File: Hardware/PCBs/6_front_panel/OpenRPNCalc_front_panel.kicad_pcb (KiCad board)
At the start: 2 copper layers, 73 x 134.4 mm, 1 part

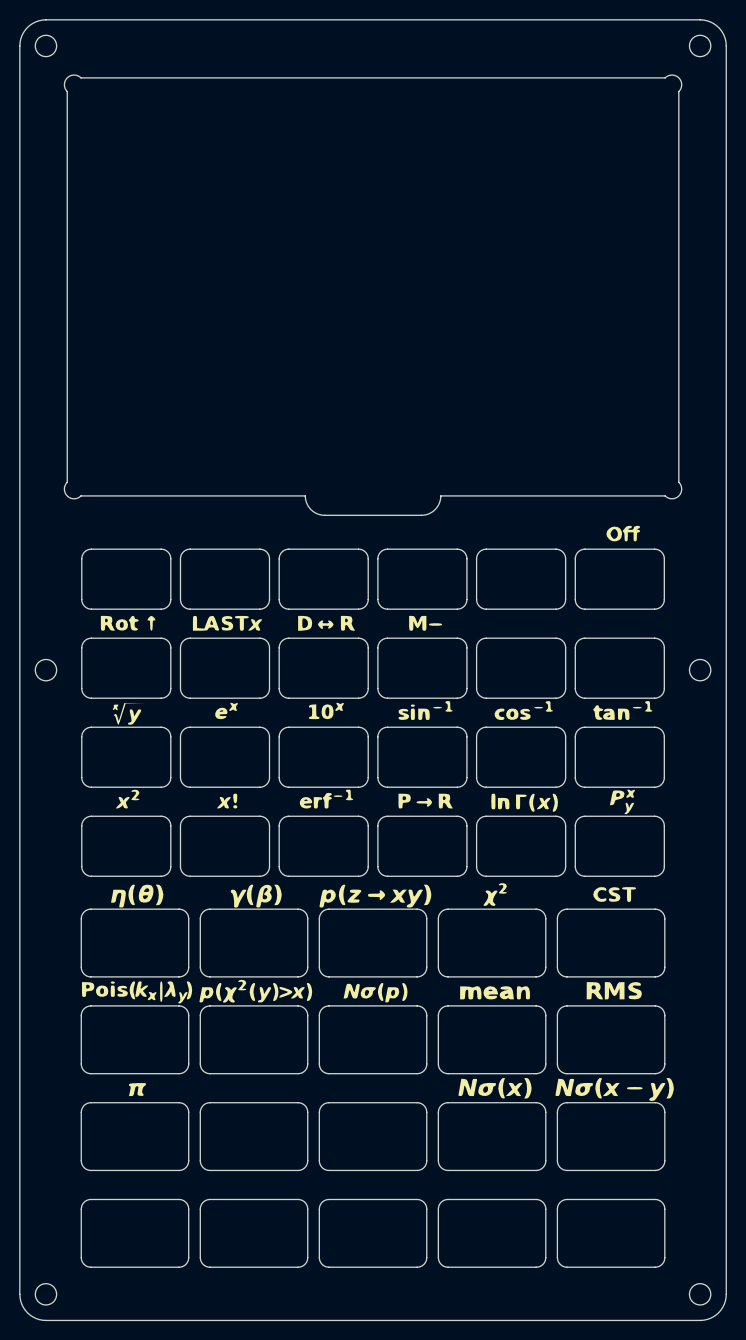
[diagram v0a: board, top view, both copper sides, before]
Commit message: Update to rev 3.1
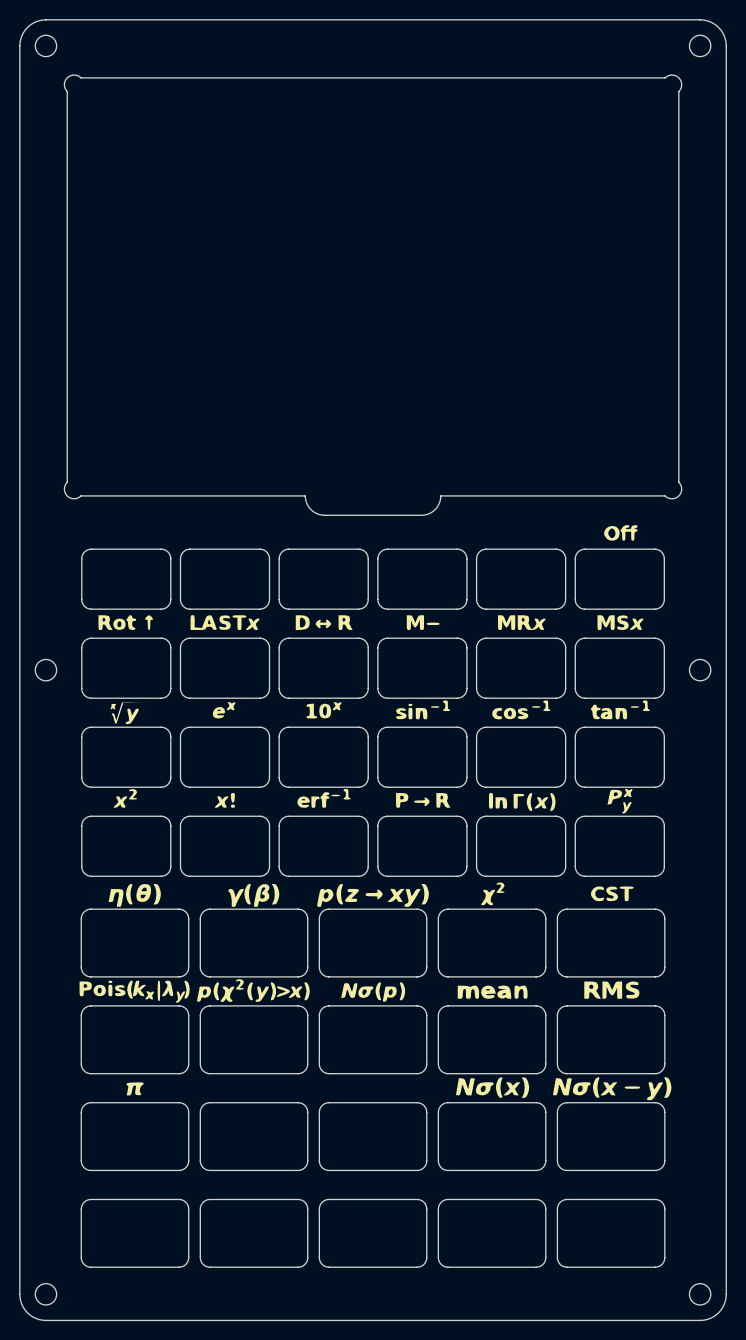
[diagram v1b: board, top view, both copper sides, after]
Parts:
- moved G*** 0.26 mm to (100.0, 97.2)

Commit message: Rev 3.1
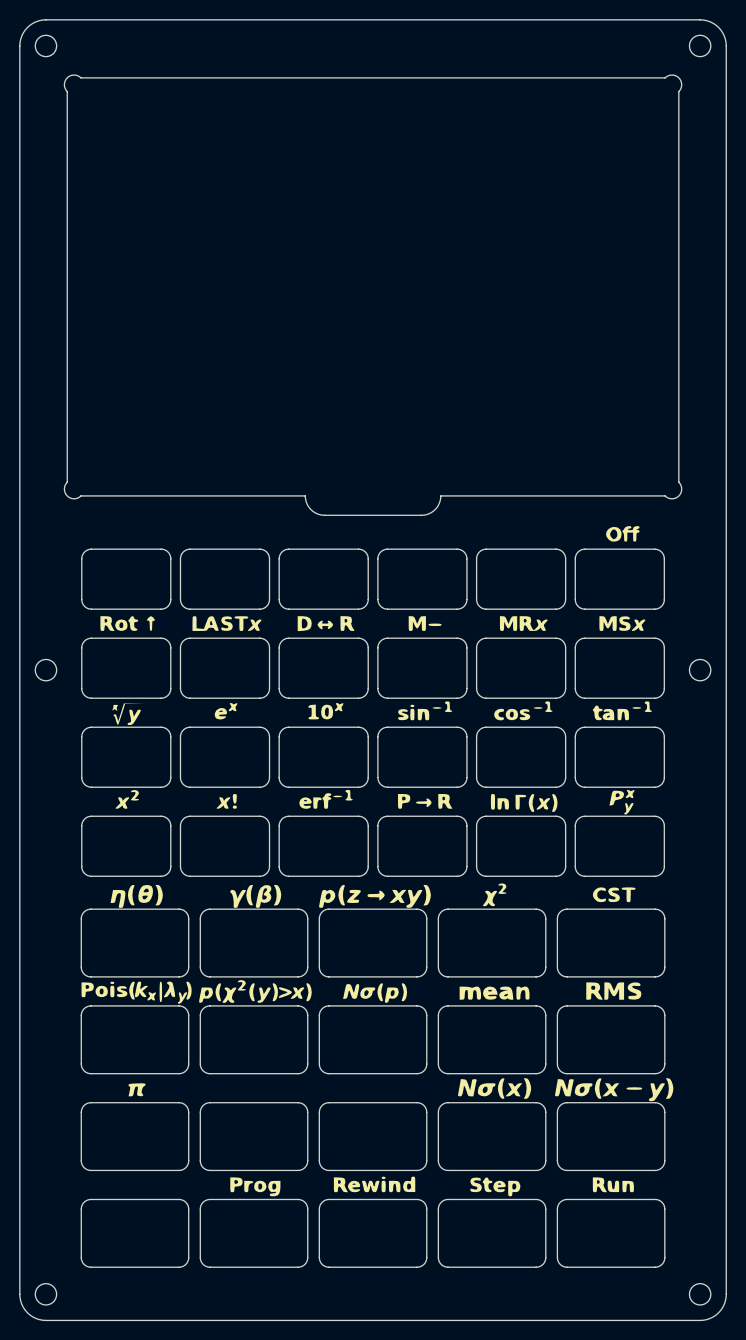
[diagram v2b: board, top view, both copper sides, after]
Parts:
- moved G*** 0.22 mm to (100.2, 97.3)
